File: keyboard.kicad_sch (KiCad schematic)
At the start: 114 parts, among them J2 TYPE-C-31-M-12, U1 ATmega32U4-A, Y1 Crystal_GND24_Small

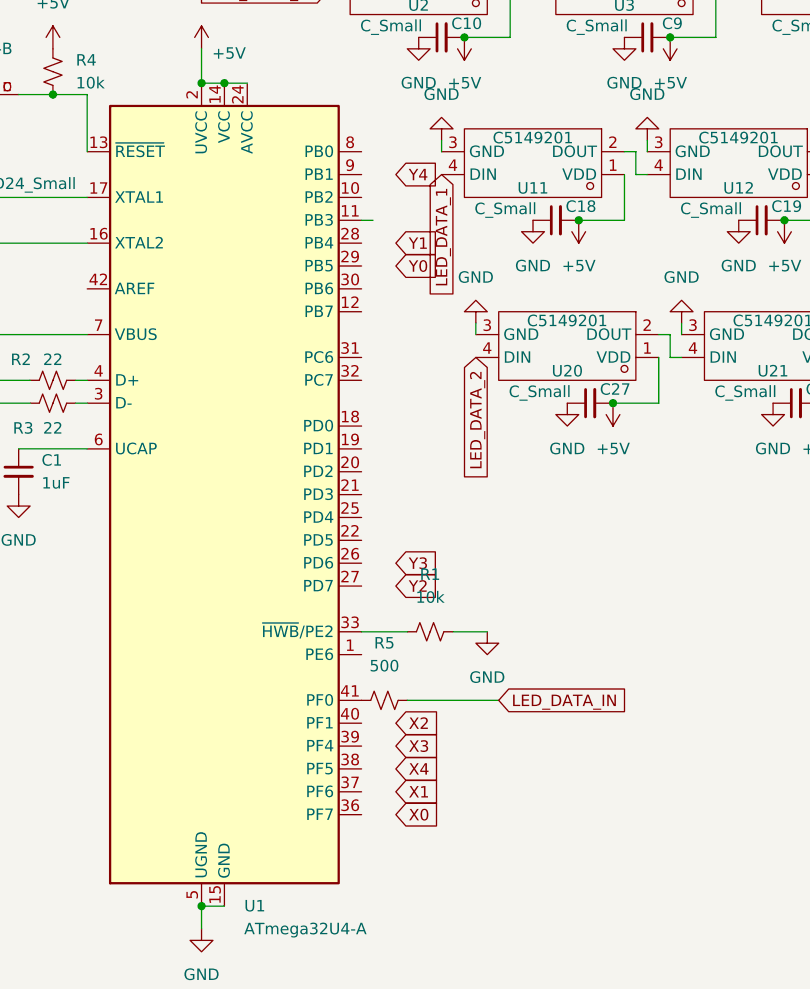
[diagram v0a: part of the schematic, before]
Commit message: upaded islands
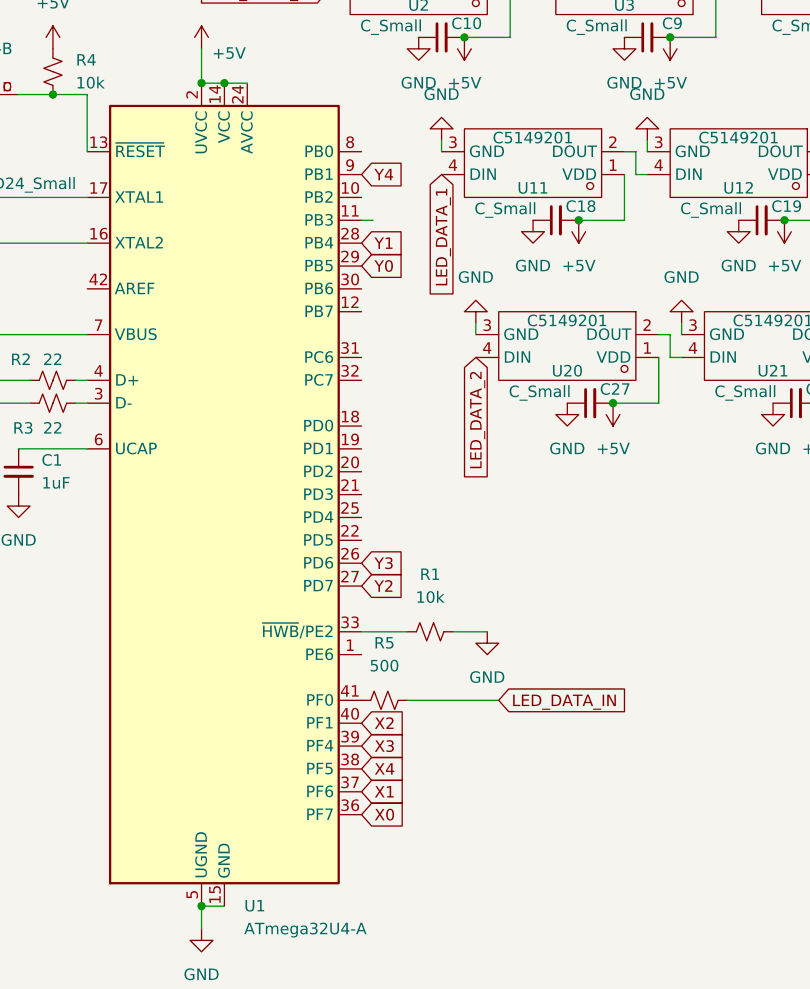
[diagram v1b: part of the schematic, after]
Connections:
- net X0: now also U1.36 (PF7)
- net X1: now also U1.37 (PF6)
- net X2: now also U1.40 (PF1)
- net X3: now also U1.39 (PF4)
- net X4: now also U1.38 (PF5)
- net Y0: now also U1.29 (PB5)
- net Y1: now also U1.28 (PB4)
- net Y2: now also U1.27 (PD7)
- net Y3: now also U1.26 (PD6)
- net Y4: now also U1.9 (PB1)
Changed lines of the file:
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@@
 	(global_label "Y2"
 		(shape input)
-		(at 82.55 86.36 0)
-		(fields_autoplaced yes)
-		(effects
-			(font
-				(size 1.27 1.27)
-			)
-			(justify left)
-		)
-		(property "Intersheetrefs" "${INTERSHEET_REFS}"
-			(at 87.8333 86.36 0)
+		(at 78.74 86.36 0)
+		(fields_autoplaced yes)
+		(effects
+			(font
+				(size 1.27 1.27)
+			)
+			(justify left)
+		)
+		(property "Intersheetrefs" "${INTERSHEET_REFS}"
+			(at 84.0233 86.36 0)
 			(effects
 				(font
@@
 	(global_label "Y1"
 		(shape input)
-		(at 82.55 48.26 0)
-		(fields_autoplaced yes)
-		(effects
-			(font
-				(size 1.27 1.27)
-			)
-			(justify left)
-		)
-		(property "Intersheetrefs" "${INTERSHEET_REFS}"
-			(at 87.8333 48.26 0)
+		(at 78.74 48.26 0)
+		(fields_autoplaced yes)
+		(effects
+			(font
+				(size 1.27 1.27)
+			)
+			(justify left)
+		)
+		(property "Intersheetrefs" "${INTERSHEET_REFS}"
+			(at 84.0233 48.26 0)
 			(effects
 				(font
@@
 	(global_label "Y3"
 		(shape input)
-		(at 82.55 83.82 0)
-		(fields_autoplaced yes)
-		(effects
-			(font
-				(size 1.27 1.27)
-			)
-			(justify left)
-		)
-		(property "Intersheetrefs" "${INTERSHEET_REFS}"
-			(at 87.8333 83.82 0)
+		(at 78.74 83.82 0)
+		(fields_autoplaced yes)
+		(effects
+			(font
+				(size 1.27 1.27)
+			)
+			(justify left)
+		)
+		(property "Intersheetrefs" "${INTERSHEET_REFS}"
+			(at 84.0233 83.82 0)
 			(effects
 				(font
@@
 	(global_label "X0"
 		(shape input)
-		(at 82.55 111.76 0)
-		(fields_autoplaced yes)
-		(effects
-			(font
-				(size 1.27 1.27)
-			)
-			(justify left)
-		)
-		(property "Intersheetrefs" "${INTERSHEET_REFS}"
-			(at 87.9542 111.76 0)
+		(at 78.74 111.76 0)
+		(fields_autoplaced yes)
+		(effects
+			(font
+				(size 1.27 1.27)
+			)
+			(justify left)
+		)
+		(property "Intersheetrefs" "${INTERSHEET_REFS}"
+			(at 84.1442 111.76 0)
 			(effects
 				(font
@@
 	(global_label "X2"
 		(shape input)
-		(at 82.55 101.6 0)
-		(fields_autoplaced yes)
-		(effects
-			(font
-				(size 1.27 1.27)
-			)
-			(justify left)
-		)
-		(property "Intersheetrefs" "${INTERSHEET_REFS}"
-			(at 87.9542 101.6 0)
+		(at 78.74 101.6 0)
+		(fields_autoplaced yes)
+		(effects
+			(font
+				(size 1.27 1.27)
+			)
+			(justify left)
+		)
+		(property "Intersheetrefs" "${INTERSHEET_REFS}"
+			(at 84.1442 101.6 0)
 			(effects
 				(font
@@
 	(global_label "Y0"
 		(shape input)
-		(at 82.55 50.8 0)
-		(fields_autoplaced yes)
-		(effects
-			(font
-				(size 1.27 1.27)
-			)
-			(justify left)
-		)
-		(property "Intersheetrefs" "${INTERSHEET_REFS}"
-			(at 87.8333 50.8 0)
+		(at 78.74 50.8 0)
+		(fields_autoplaced yes)
+		(effects
+			(font
+				(size 1.27 1.27)
+			)
+			(justify left)
+		)
+		(property "Intersheetrefs" "${INTERSHEET_REFS}"
+			(at 84.0233 50.8 0)
 			(effects
 				(font
@@
 	(global_label "X1"
 		(shape input)
-		(at 82.55 109.22 0)
-		(fields_autoplaced yes)
-		(effects
-			(font
-				(size 1.27 1.27)
-			)
-			(justify left)
-		)
-		(property "Intersheetrefs" "${INTERSHEET_REFS}"
-			(at 87.9542 109.22 0)
+		(at 78.74 109.22 0)
+		(fields_autoplaced yes)
+		(effects
+			(font
+				(size 1.27 1.27)
+			)
+			(justify left)
+		)
+		(property "Intersheetrefs" "${INTERSHEET_REFS}"
+			(at 84.1442 109.22 0)
 			(effects
 				(font
@@
 	(global_label "X3"
 		(shape input)
-		(at 82.55 104.14 0)
-		(fields_autoplaced yes)
-		(effects
-			(font
-				(size 1.27 1.27)
-			)
-			(justify left)
-		)
-		(property "Intersheetrefs" "${INTERSHEET_REFS}"
-			(at 87.9542 104.14 0)
+		(at 78.74 104.14 0)
+		(fields_autoplaced yes)
+		(effects
+			(font
+				(size 1.27 1.27)
+			)
+			(justify left)
+		)
+		(property "Intersheetrefs" "${INTERSHEET_REFS}"
+			(at 84.1442 104.14 0)
 			(effects
 				(font
@@
 	(global_label "Y4"
 		(shape input)
-		(at 82.55 40.64 0)
-		(fields_autoplaced yes)
-		(effects
-			(font
-				(size 1.27 1.27)
-			)
-			(justify left)
-		)
-		(property "Intersheetrefs" "${INTERSHEET_REFS}"
-			(at 87.8333 40.64 0)
+		(at 78.74 40.64 0)
+		(fields_autoplaced yes)
+		(effects
+			(font
+				(size 1.27 1.27)
+			)
+			(justify left)
+		)
+		(property "Intersheetrefs" "${INTERSHEET_REFS}"
+			(at 84.0233 40.64 0)
 			(effects
 				(font
@@
 	(global_label "X4"
 		(shape input)
-		(at 82.55 106.68 0)
-		(fields_autoplaced yes)
-		(effects
-			(font
-				(size 1.27 1.27)
-			)
-			(justify left)
-		)
-		(property "Intersheetrefs" "${INTERSHEET_REFS}"
-			(at 87.9542 106.68 0)
-			(effects
-				(font
+		(at 78.74 106.68 0)
+		(fields_autoplaced yes)
+		(effects
+			(font
+				(size 1.27 1.27)
+			)
+			(justify left)
+		)
+		(property "Intersheetrefs" "${INTERSHEET_REFS}"
+			(at 84.1442 106.68 0)
+			(effects
+				(font
